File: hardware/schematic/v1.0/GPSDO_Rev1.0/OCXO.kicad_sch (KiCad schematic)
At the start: 31 parts, among them U2 LMK1C1103PWR, U3 TMP117AIDRVR, U5 OCXO_20x20mm, U7 OCXO_25.4x25.4mm, U8 REF5040

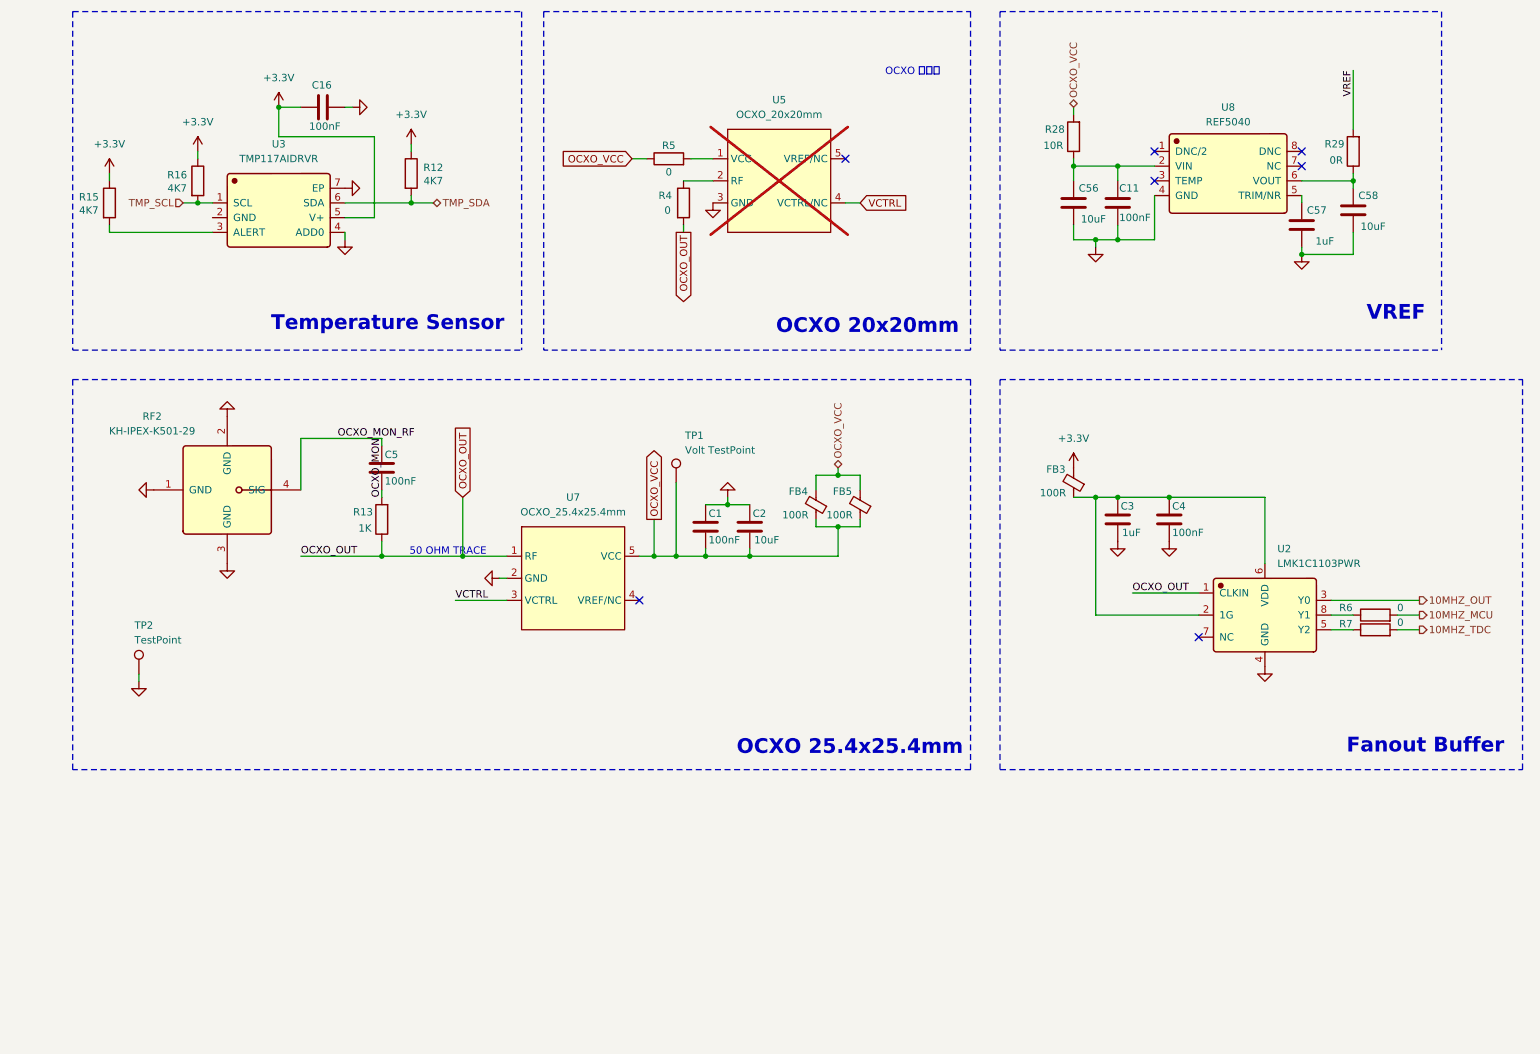
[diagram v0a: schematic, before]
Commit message: sch update
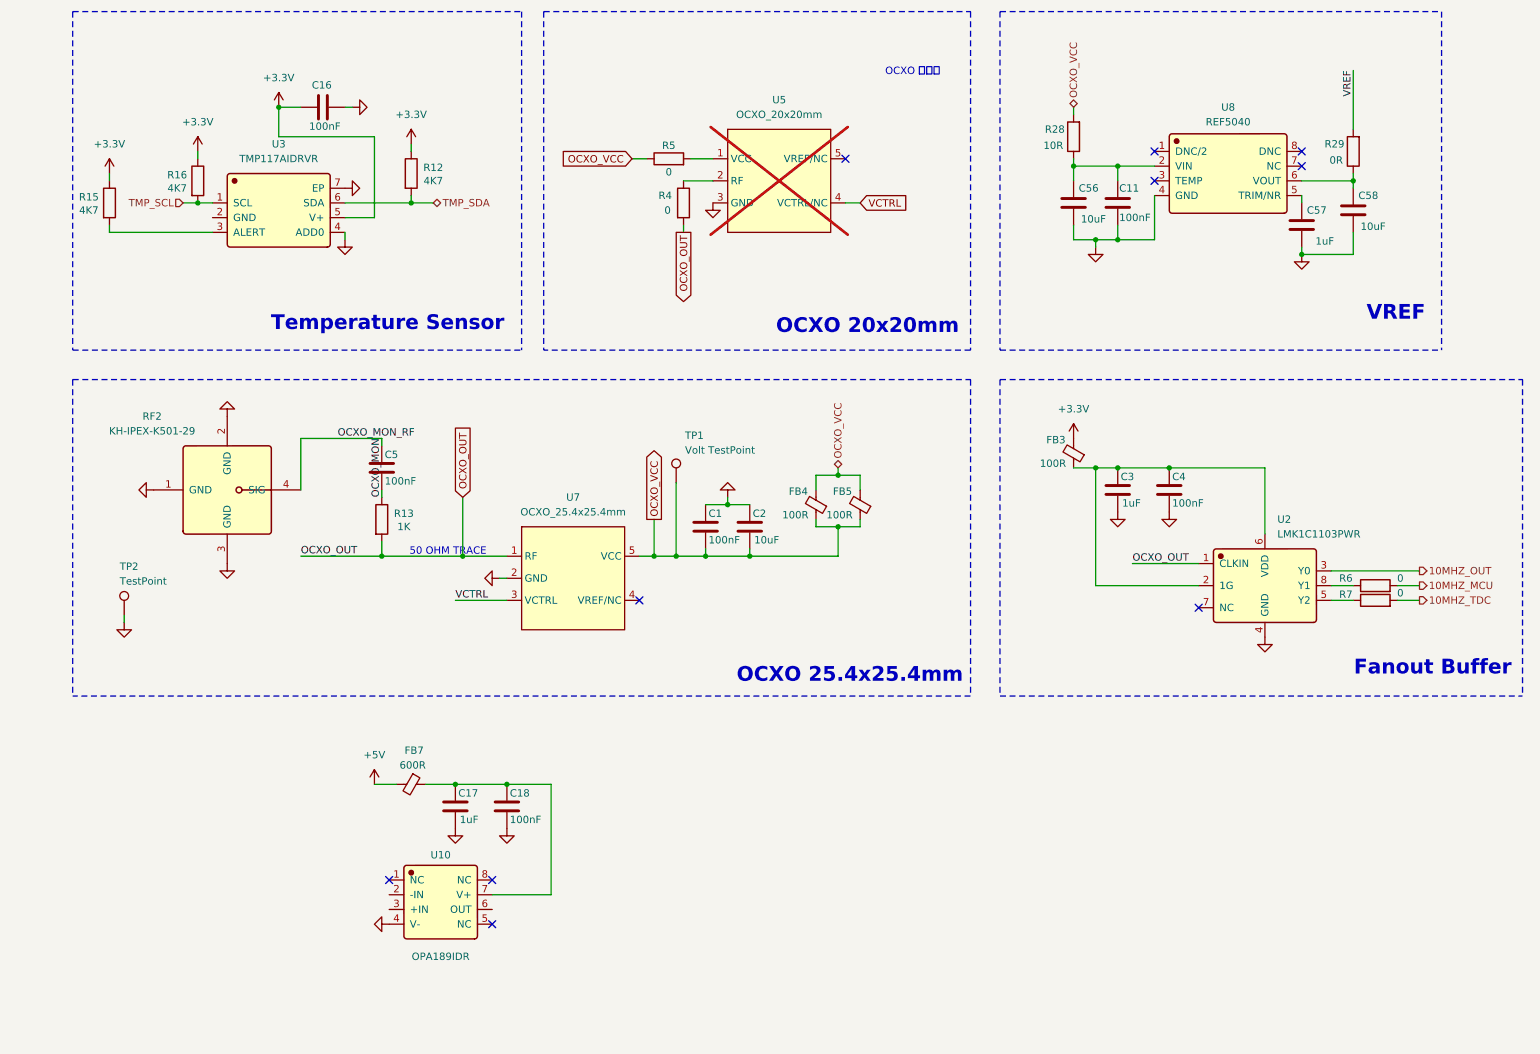
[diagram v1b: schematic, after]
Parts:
- removed R13: 1K, Resistor_SMD:R_0402_1005Metric, symbol Device:R
- added C17: 1uF, GPSDO_Rev1.0:C_0603_1608Metric, symbol GPSDO_Rev1.0:C
- added C18: 100nF, GPSDO_Rev1.0:C_0402_1005Metric, symbol GPSDO_Rev1.0:C
- added FB7: 600R, GPSDO_Rev1.0:L_0603_1608Metric, symbol GPSDO_Rev1.0:FerriteBead_Small
- added R13: 1K, GPSDO_Rev1.0:R_0402_1005Metric, symbol GPSDO_Rev1.0:R
- added U10: OPA189IDR, GPSDO_Rev1.0:OPA189IDR, symbol GPSDO_Rev1.0:OPA189IDR
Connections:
- net GND: now also C17.2, C18.2, U10.4 (V-)
- net OCXO_MON: now also R13.1
- net OCXO_OUT: now also R13.2
- new net: C17.1, C18.1, FB7.1, U10.7 (V+)
- new net +5V: FB7.2
- no-connect marks 7 -> 10
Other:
- moved on the sheet: C3, C4, FB3, R6, R7, TP2, U2

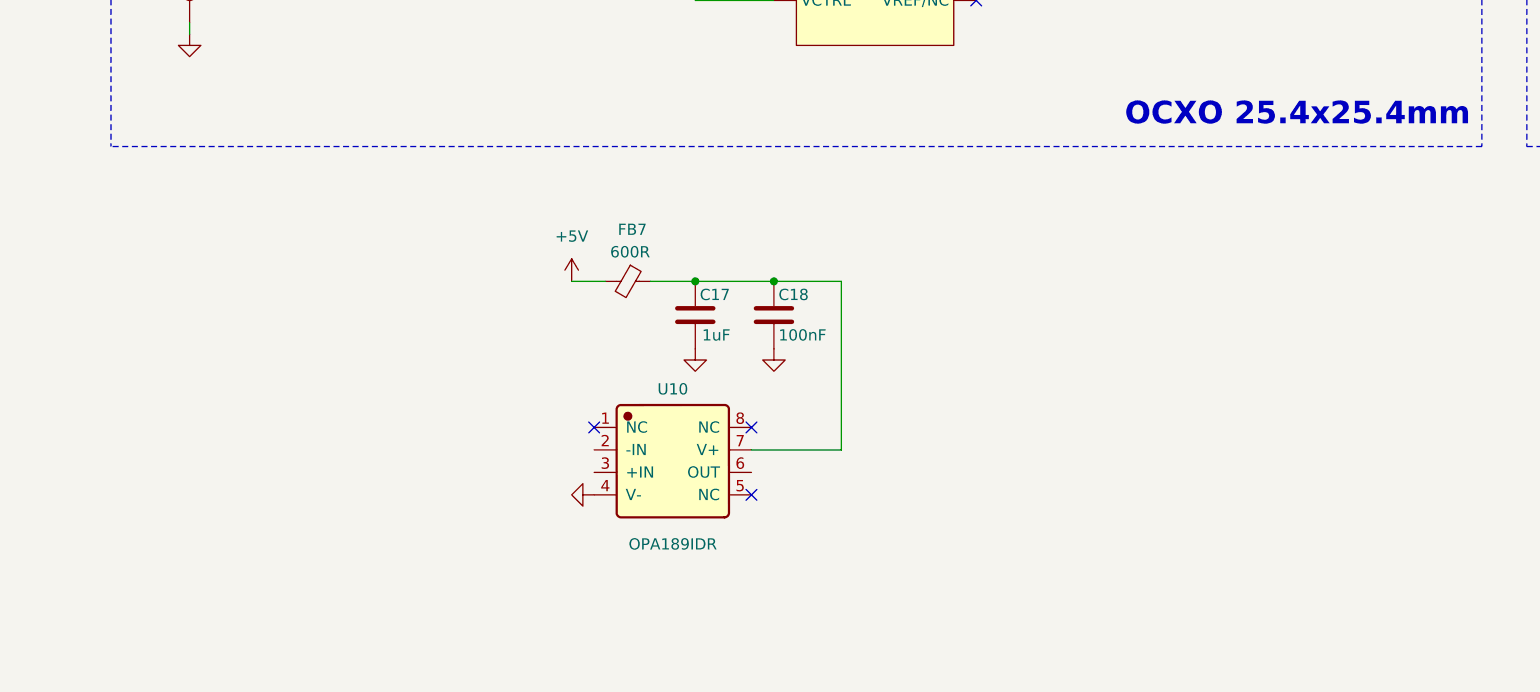
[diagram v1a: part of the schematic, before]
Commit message: sch update
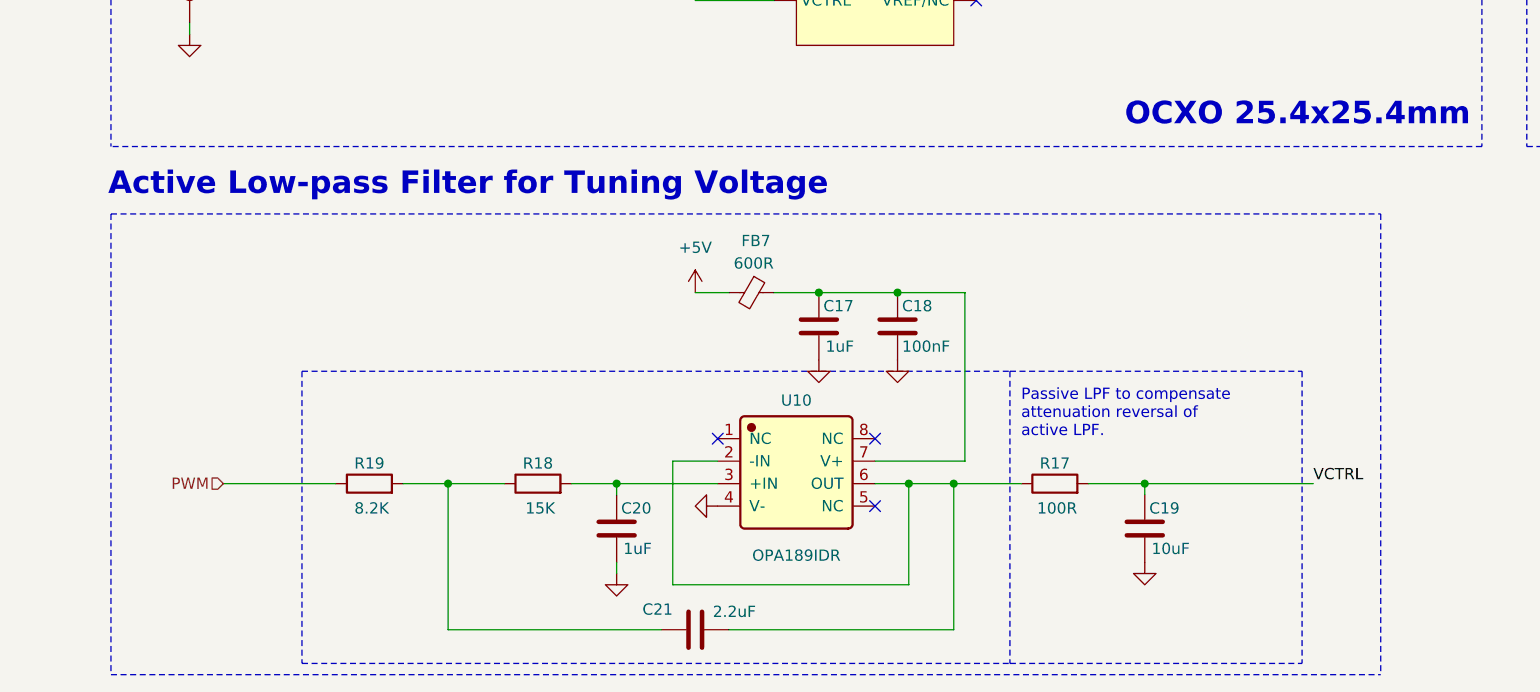
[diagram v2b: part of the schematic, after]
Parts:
- added C19: 10uF, GPSDO_Rev1.0:C_0603_1608Metric, symbol GPSDO_Rev1.0:C
- added C20: 1uF, GPSDO_Rev1.0:C_0603_1608Metric, symbol GPSDO_Rev1.0:C
- added C21: 2.2uF, GPSDO_Rev1.0:C_0603_1608Metric, symbol GPSDO_Rev1.0:C
- added R17: 100R, GPSDO_Rev1.0:R_0603_1608Metric, symbol GPSDO_Rev1.0:R
- added R18: 15K, GPSDO_Rev1.0:R_0603_1608Metric, symbol GPSDO_Rev1.0:R
- added R19: 8.2K, GPSDO_Rev1.0:R_0603_1608Metric, symbol GPSDO_Rev1.0:R
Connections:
- net GND: now also C19.2, C20.2
- net VCTRL: now also C19.1, R17.2
- net at U10.2 (-IN): now also U10.6 (OUT), C21.2, R17.1
- net at U10.3 (+IN): now also C20.1, R18.2
- new net: C21.1, R18.1, R19.2
- new net PWM: R19.1
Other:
- note added: "Active Low-pass Filter for Tuning Voltage"
- note added: "Passive LPF to compensate attenuation reversal of active LPF."
- moved on the sheet: C17, C18, FB7, U10

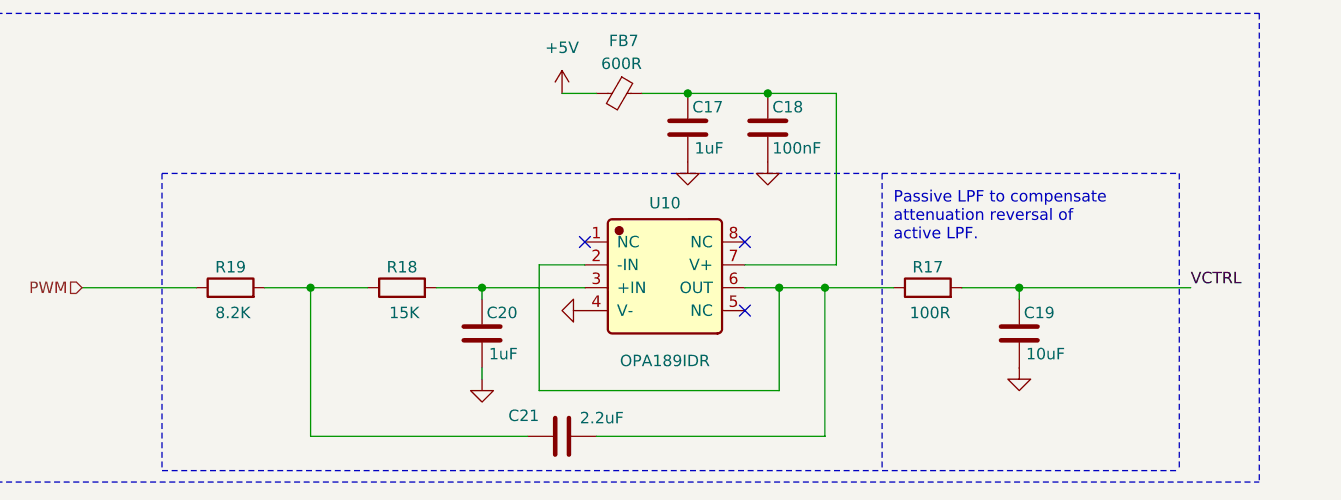
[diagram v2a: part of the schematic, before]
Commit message: sch update
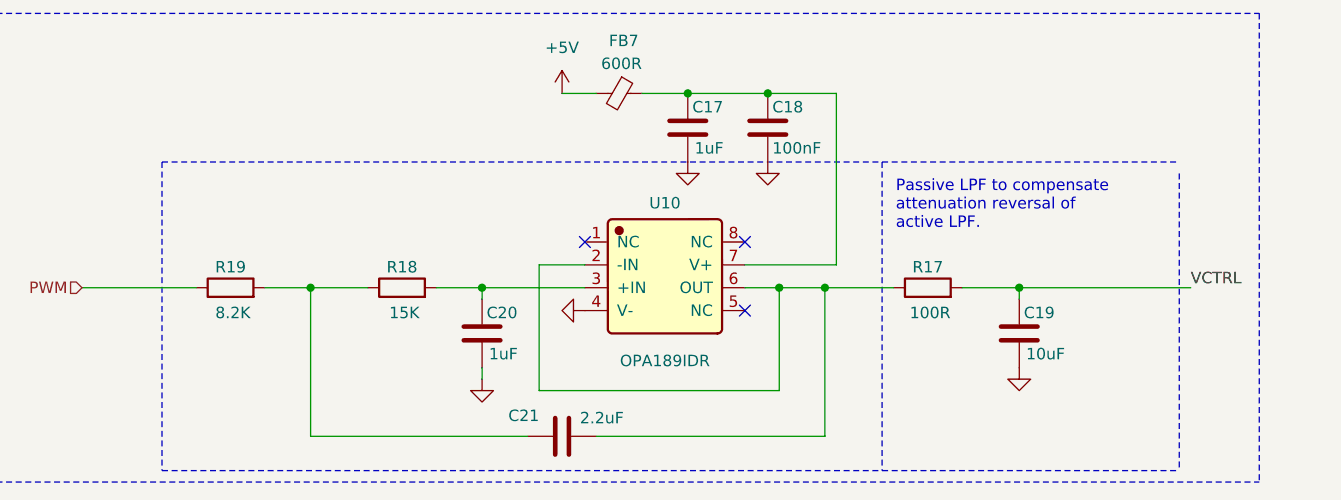
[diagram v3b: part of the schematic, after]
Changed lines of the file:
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@@
 	(text "Passive LPF to compensate\nattenuation reversal of \nactive LPF."
 		(exclude_from_sim no)
-		(at 128.27 166.116 0)
+		(at 128.524 164.846 0)
 		(effects
 			(font
@@
 	(polyline
 		(pts
-			(xy 127 161.29) (xy 127 194.31)
+			(xy 127 160.02) (xy 127 194.31)
 		)
 		(stroke
@@
 	(polyline
 		(pts
-			(xy 46.99 161.29) (xy 46.99 194.31)
+			(xy 46.99 160.02) (xy 46.99 194.31)
 		)
 		(stroke
@@
 	(polyline
 		(pts
-			(xy 46.99 161.29) (xy 127 161.29)
+			(xy 46.99 160.02) (xy 127 160.02)
 		)
 		(stroke
@@
 	(polyline
 		(pts
-			(xy 127 161.29) (xy 160.02 161.29)
-		)
-		(stroke
+			(xy 127 160.02) (xy 160.02 160.02)
+		)
+		(stroke
